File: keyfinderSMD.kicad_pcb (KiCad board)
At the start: 2 copper layers, 22 parts, among them Q1 2N7002, U1 4049

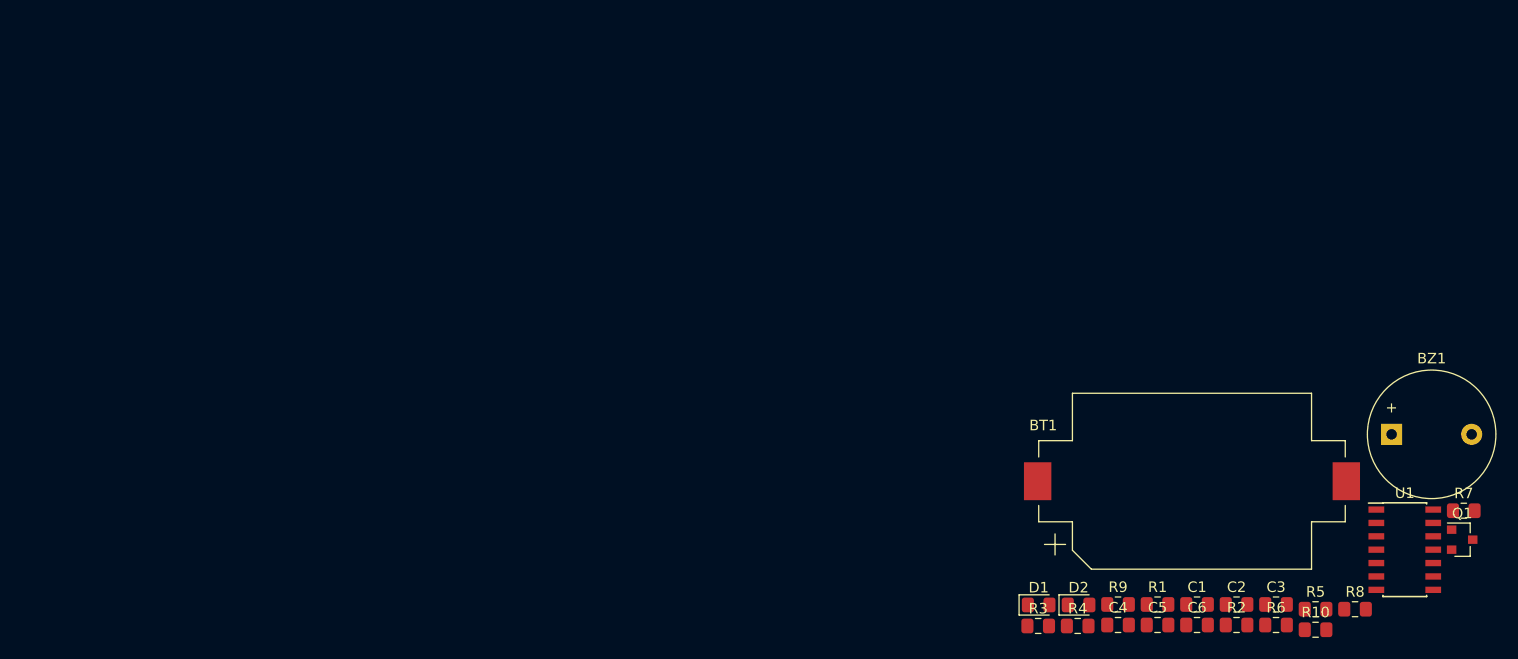
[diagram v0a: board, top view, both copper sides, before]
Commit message: added first draft
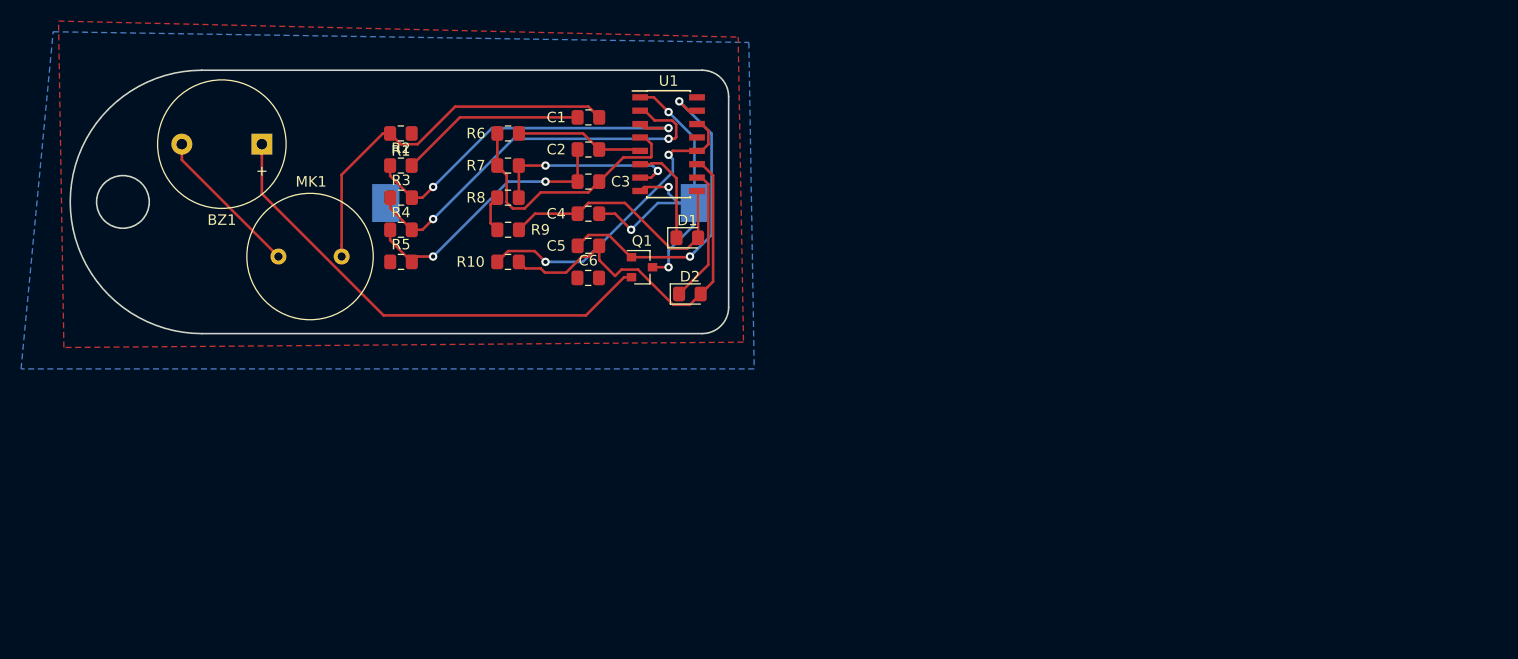
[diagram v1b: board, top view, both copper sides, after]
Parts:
- added MK1: Microphone, keyfinderSMD:MicrophoneDIP, F.Cu at (80.3, 75.2)
- BT1: moved to B.Cu
- BZ1: footprint Buzzer_Beeper:Buzzer_12x9.5RM7.6 -> keyfinderSMD:Buzzer_12x9.5RM7.6
- U1: footprint Package_SO:SOIC-14_3.9x8.7mm_P1.27mm -> Package_SO:SOIC-16_3.9x9.9mm_P1.27mm
- moved BZ1 110.7 mm to (75.7, 64.5), turned to 180 degrees
- moved R7 96.5 mm to (99.1, 66.5), turned to 180 degrees
- moved R5 92.9 mm to (88.9, 75.7)
- moved R2 90.5 mm to (88.9, 66.5)
- moved R8 89.4 mm to (99.1, 69.6)
- moved R6 86.6 mm to (99.1, 63.5)
- moved R1 84.6 mm to (88.9, 63.5), turned to 180 degrees
- moved R10 84.2 mm to (99.1, 75.7)
- moved Q1 82.0 mm to (111.8, 76.2)
- moved U1 79.8 mm to (114.3, 64.5)
- moved C3 76.6 mm to (106.7, 68.1), turned to 180 degrees
- moved C2 75.2 mm to (106.7, 65.0)
- moved R4 74.4 mm to (88.9, 72.6)
- moved C1 74.0 mm to (106.7, 62.0)
- moved R3 72.9 mm to (88.9, 69.6)
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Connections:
- BT1 pad 1: GND -> +3V3
- BT1 pad 2: GND -> VS
- BZ1 pad 2: GND -> VS
- C4 pad 2: GND -> VS
- C6 pad 1: GND -> VS
- C6 pad 2: GND -> VS
- Q1 pad 3: GND -> VS
- R1 pad 1: GND -> VS
- R5 pad 1: GND -> VS
- R8 pad 1: GND -> VS
- R9 pad 2: GND -> VS
- U1 pad 1: GND -> VS
- U1 pad 8: GND -> VS
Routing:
- net VS: track 0.00 -> 56.6 mm, vias 0 -> 4
- net Net-(BZ1-Pad1): track 0.00 -> 46.1 mm
- net Net-(R3-Pad1): track 0.00 -> 37.8 mm, vias 0 -> 2
- net Net-(C5-Pad2): track 0.00 -> 36.5 mm
- net Net-(C1-Pad2): track 0.00 -> 36.2 mm
- net Net-(R2-Pad1): track 0.00 -> 33.9 mm, vias 0 -> 2
- net Net-(C5-Pad1): track 0.00 -> 30.9 mm, vias 0 -> 2
- net Net-(R10-Pad1): track 0.00 -> 29.7 mm, vias 0 -> 2
- net Net-(C2-Pad1): track 0.00 -> 25.8 mm, vias 0 -> 2
- net Net-(C3-Pad1): track 0.00 -> 25.5 mm
- net Net-(C4-Pad1): track 0.00 -> 24.8 mm
- net Net-(R7-Pad1): track 0.00 -> 18.4 mm, vias 0 -> 2
- net Net-(C1-Pad1): track 0.00 -> 17.6 mm
- net Net-(D2-Pad1): track 0.00 -> 12.9 mm
- net Net-(C2-Pad2): track 0.00 -> 12.2 mm
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- added copper zone on B.Cu, net VS
- added copper zone on F.Cu, net VS
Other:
- board outline added: 62.5 x 25 mm
